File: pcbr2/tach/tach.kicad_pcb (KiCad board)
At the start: 2 copper layers, 51 x 52.9 mm, 90 parts, among them J1 Screw_Terminal_01x02, J2 Conn_01x01, J3 Conn_01x01, J4 XF2M-1415-1A, J5 FTSH-105-01-L-DV-007-K, J6 Conn_01x01, J7 Conn_01x01, Q1 MMBT3904-7-F, Q2 MMBT3906-7-F, U1 TMP20AIDCK, U10 X27.589, U2 TLV6001, U3 LTC2053, U4 LM2840X, U5 LM2937xMP-3.3, U6 STM32F103CBTx, U7 LM27762, U8 74ABT126, Y1 16MHz

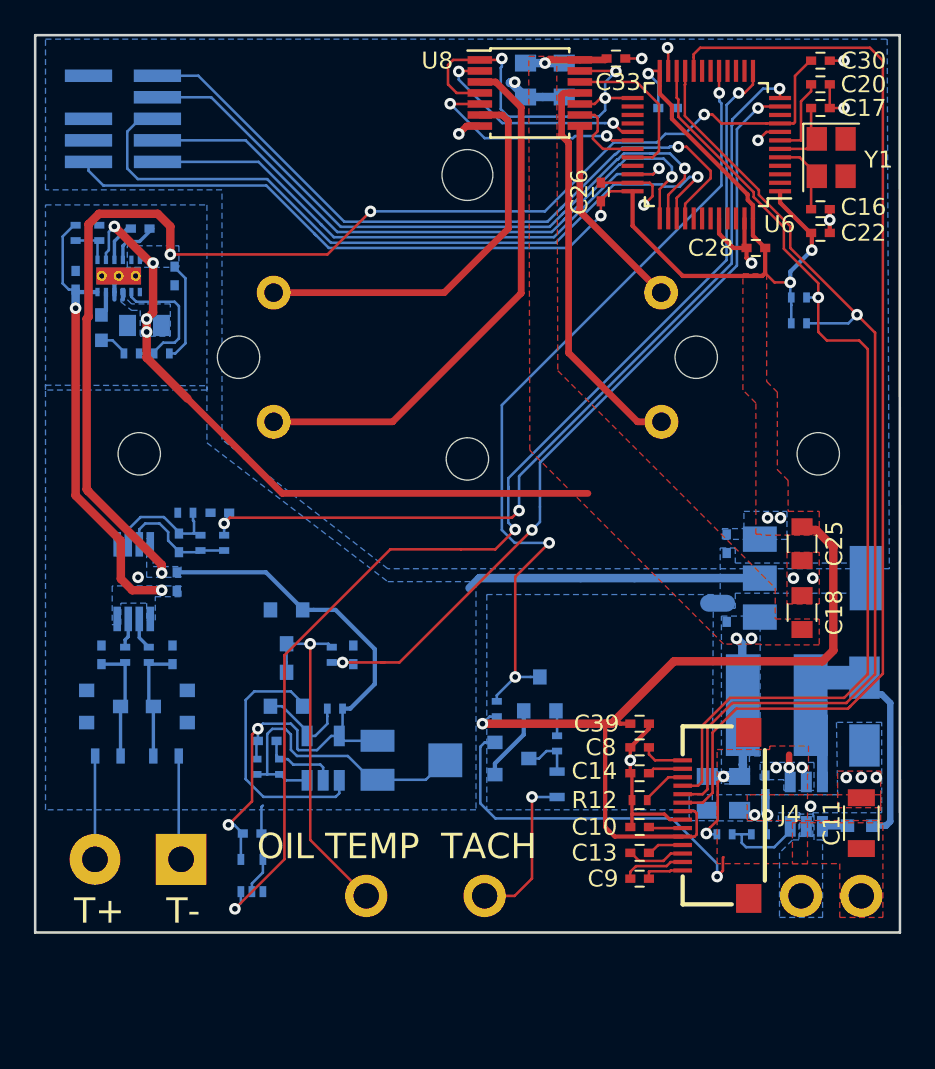
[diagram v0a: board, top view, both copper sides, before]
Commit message: this commit preserves the state of the repo as of 7/13/26. confirmed working in hardware.
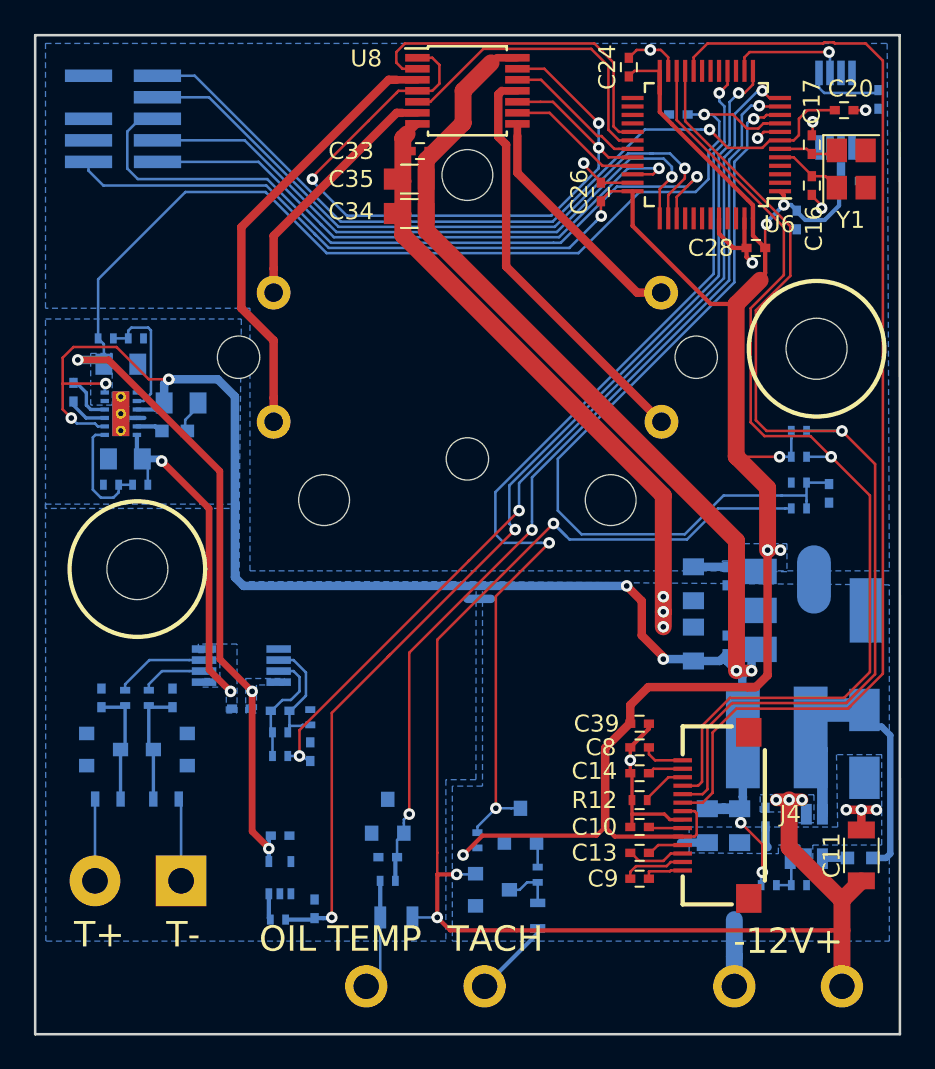
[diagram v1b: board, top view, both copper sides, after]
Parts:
- removed Q2: MMBT3906-7-F, TO_SOT_Packages_SMD:SOT-23
- removed RV1: 100k, Potentiometers:Potentiometer_Trimmer_Bourns_3224J
- added C40: 0.1/10, Capacitors_SMD:C_0402, B.Cu at (175.5, 73.3)
- added C41: 1.0/10, Capacitors_SMD:C_0402, B.Cu at (177.2, 68.5)
- added C42: 0.01/10, Capacitors_SMD:C_0402, B.Cu at (174.2, 91.7)
- added R21: 18.2k 0.1%, Resistors_SMD:R_0402, B.Cu at (172.5, 91.1)
- C18, C22, C25: moved to B.Cu
- C24, C34, C35: moved to F.Cu
- C3: value 0.01u/25 -> 0.01/25
- C30: value 0.1/10 -> 1.0/10; moved to B.Cu
- C36, C37: footprint Capacitors_SMD:C_0402 -> Capacitors_SMD:C_0805
- C4: value 0.1/16 -> 0.01/10
- D2: value BAS40-04 -> SZMMBZ5222BLT1G
- H1, H2: footprint Mounting_Holes:MountingHole_2.5mm -> footprints:MountingHole_M3
- R1: value 22k -> 10k
- R2: value 100k -> 2.2k 0.1%; footprint Resistors_SMD:R_0402 -> Resistors_SMD:R_0805
- R5: value 100 -> 10k
- R8: value 10k -> 80.6k 0.1%
- U2: value TLV6001 -> REF5025ADGK; footprint TO_SOT_Packages_SMD:TSOT-23-5 -> Housings_SSOP:MSOP-8_3x3mm_Pitch0.65mm
- moved U2 48.7 mm to (174.6, 69.1)
- moved R8 28.9 mm to (172.5, 92.6), turned to 0 degrees
- moved R18 15.3 mm to (133.6, 91.2), turned to 0 degrees
- moved C12 15.1 mm to (143.6, 106.9), turned to 90 degrees
- moved R20 14.9 mm to (131.9, 91.2), turned to 0 degrees
- moved R10 14.1 mm to (143.6, 104.9), turned to 90 degrees
- moved R11 13.0 mm to (141.9, 107.2), turned to 180 degrees
- moved C33 12.8 mm to (150.1, 71.5), turned to 180 degrees
- moved D2 12.7 mm to (148.2, 110.7), turned to 90 degrees
- moved R9 12.1 mm to (141.9, 105.8), turned to 0 degrees
- moved C5 12.1 mm to (148.2, 113.2), turned to 180 degrees
- moved C7 11.6 mm to (141.9, 104.5), turned to 0 degrees
- moved R2 11.2 mm to (148.7, 116.7), turned to 180 degrees
- moved C37 10.9 mm to (132.7, 89.7), turned to 0 degrees
- moved C35 10.9 mm to (149.5, 73.2), turned to 180 degrees
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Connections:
- C4 pad 1: /+3.3VA -> /COLD_JUNC
- D2 pad 1: GND -> /OIL_TEMP
- D2 pad 2: /+3.3VA -> GND
- D2 pad 3: /OIL_TEMP_IN -> (no net)
- J5 pad 10: /JNTRST -> /NRST
- R1 pad 1: /+3.3VA -> /COLD_JUNC
- R2 pad 1: Net-(R1-Pad2) -> +12V
- R2 pad 2: GND -> /OIL_TEMP_IN
- R5 pad 1: /+3.3VA -> /OIL_TEMP
- R5 pad 2: Net-(Q2-Pad2) -> /OIL_TEMP_IN
- R8 pad 1: /OIL_TEMP -> +12V
- R8 pad 2: /OIL_TEMP_IN -> /BATT_SENS
- U1 pad 3: /COLD_JUNC -> Net-(R1-Pad2)
- U2 pad 2: GND -> +3V3
- U2 pad 3: Net-(R1-Pad2) -> Net-(U2-Pad3)
- U2 pad 4: Net-(Q2-Pad2) -> GND
- U2 pad 5: /+3.3VA -> Net-(C41-Pad1)
- U6 pad 10: Net-(U6-Pad10) -> /BATT_SENS
- U6 pad 14: Net-(U6-Pad14) -> /2V5_REF
- U6 pad 16: Net-(U6-Pad16) -> /TACH
- U6 pad 17: /TACH -> Net-(U6-Pad17)
- U6 pad 25: /STEPPER_EN -> Net-(U6-Pad25)
- U6 pad 31: /STEPPER2 -> /STEPPER1
- U6 pad 32: /STEPPER1 -> /STEPPER_EN
- U6 pad 33: Net-(U6-Pad33) -> /STEPPER2
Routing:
- net +5V: track 63.5 -> 132.2 mm
- net +12V: track 23.5 -> 86.6 mm, vias 4 -> 6
- net /BATT_SENS: track 0.00 -> 48.9 mm, vias 0 -> 1
- net /NRST: track 4.79 -> 47.7 mm, vias 0 -> 1
- net /JNTRST: track 42.7 -> 0.00 mm, vias 1 -> 0
- net /+3.3VA: track 119.7 -> 95.0 mm, vias 6 -> 4
- net /STEPPER_EN: track 24.5 -> 48.3 mm
- net +3V3: track 123.7 -> 143.9 mm
- net Net-(R1-Pad2): track 18.4 -> 1.56 mm
- net Net-(U2-Pad1): track 15.4 -> 0.00 mm
- net /OIL_TEMP_IN: track 20.7 -> 6.57 mm, vias 1 -> 0
- net /TACH: track 47.7 -> 57.0 mm
- net GND: track 71.9 -> 81.0 mm, vias 20 -> 14
- net Net-(U10-Pad3): track 23.6 -> 14.8 mm
- net /OIL_TEMP: track 47.7 -> 56.2 mm
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- removed copper zone on F.Cu, net +12V
- removed copper zone on F.Cu, net +3V3
- removed copper zone on B.Cu, net +5V
- removed copper zone on F.Cu, net +5V
- removed copper zone on F.Cu, net GND
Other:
- board size 51 x 52.9 mm -> 51 x 58.9 mm
- board text added: "-12V+"
